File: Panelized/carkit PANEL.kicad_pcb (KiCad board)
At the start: 2 copper layers, 100 x 92 mm, 110 parts, among them J1 Barrel_Jack, J10 Conn_02x03_Odd_Even, J11 Conn_01x02_Pin, J12 Conn_01x02_Pin, J2 Conn_01x02_Pin, J3 Conn_02x03_Odd_Even, J4 Conn_02x03_Odd_Even, J5 Conn_01x02_Pin, J6 Conn_01x02_Pin, J7 Barrel_Jack, J8 Conn_01x02_Pin, J9 Conn_02x03_Odd_Even, P1 USB_C_Plug, P2 USB_C_Plug, SW1 SW_Push, SW2 SW_Push, SW3 SW_Push, SW4 SW_Push, U1 ESP32-C3-MINI-1, U10 DRV8876PWPR, U2 LM2596SX-5.0/NOPB, U3 AMS1117-3.3, U4 DRV8876PWPR, U5 DRV8876PWPR, U6 ESP32-C3-MINI-1, U7 LM2596SX-5.0/NOPB, U8 AMS1117-3.3, U9 DRV8876PWPR

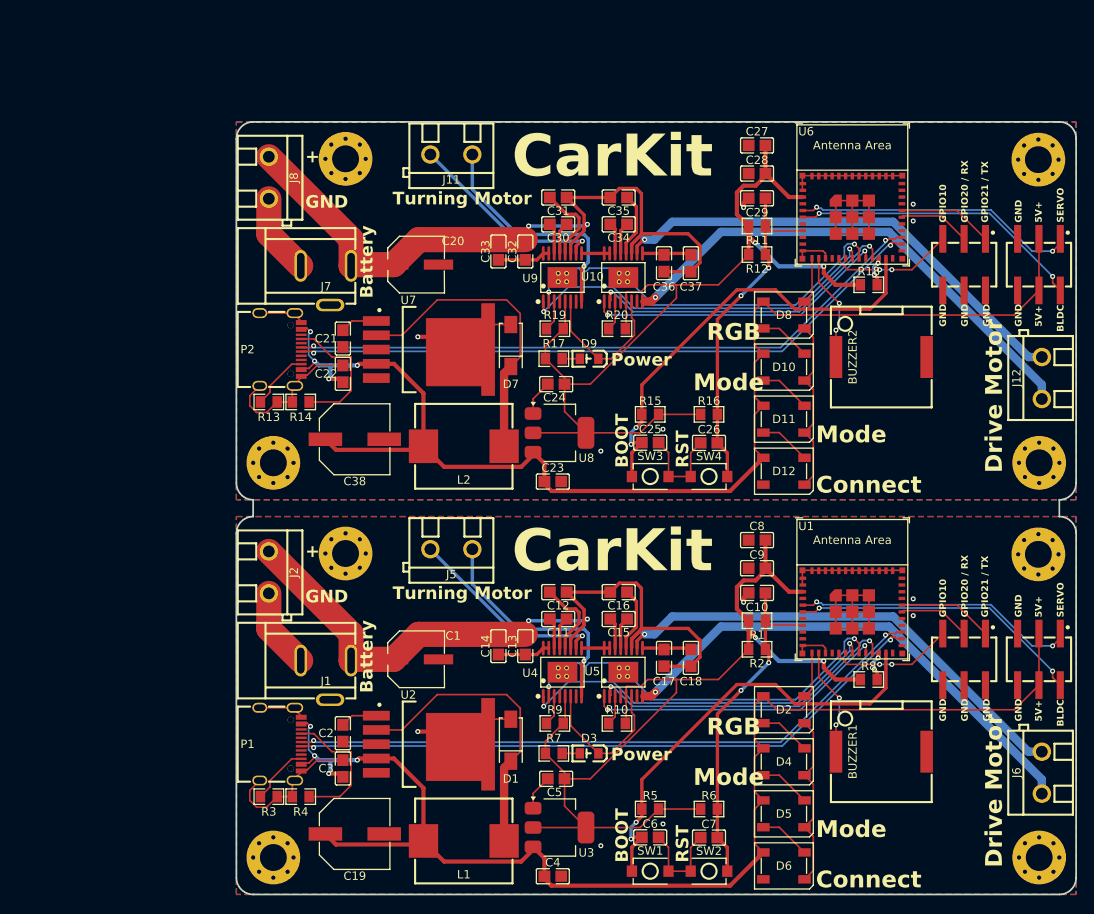
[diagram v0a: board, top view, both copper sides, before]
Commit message: Panelization Complete
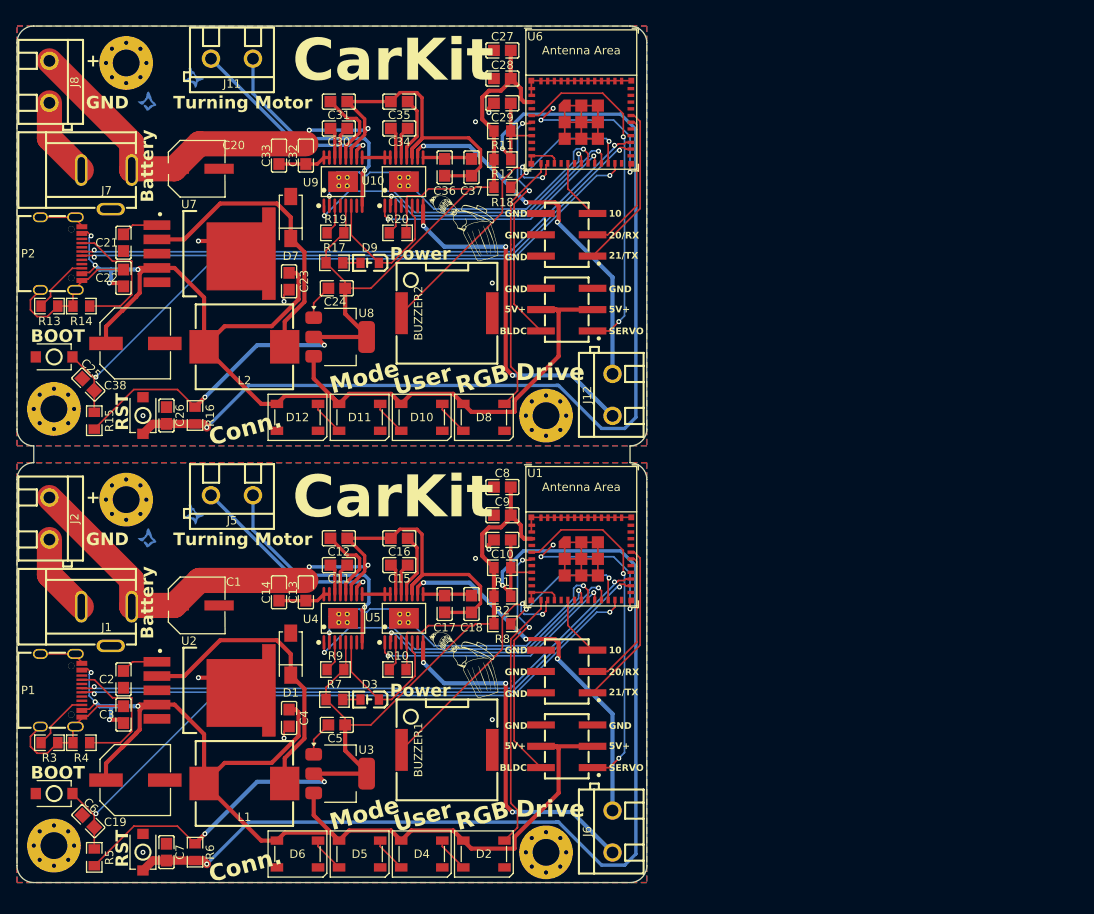
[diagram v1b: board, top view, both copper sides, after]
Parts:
- removed H7, H8: MountingHole, MountingHole:MountingHole_3.2mm_M3_Pad_Via
- added G***: LOGO, LOGO, F.Cu at (117.9, 106.2)
- added G***: LOGO, LOGO, B.Cu at (96.0, 122.6)
- added G***: LOGO, LOGO, B.Cu at (129.3, 94.3)
- added G***: LOGO, LOGO, B.Cu at (102.9, 90.8)
- added G***: LOGO, LOGO, B.Cu at (89.3, 99.5)
- added G***: LOGO, LOGO, B.Cu at (119.6, 114.5)
- added G***: LOGO, LOGO, B.Cu at (115.3, 91.4)
- added G***: LOGO, LOGO, B.Cu at (78.9, 118.2)
- added G***1: LOGO, LOGO, B.Cu at (96.0, 70.6)
- added G***2: LOGO, LOGO, B.Cu at (78.9, 66.2)
- added G***3: LOGO, LOGO, B.Cu at (119.6, 62.5)
- added G***4: LOGO, LOGO, F.Cu at (117.9, 54.2)
- added G***5: LOGO, LOGO, B.Cu at (89.3, 47.5)
- added G***6: LOGO, LOGO, B.Cu at (129.3, 42.3)
- added G***7: LOGO, LOGO, B.Cu at (115.3, 39.4)
- added G***8: LOGO, LOGO, B.Cu at (102.9, 38.8)
- moved H4 128.9 mm to (68.9, 75.4)
- moved SW3 72.4 mm to (69.0, 69.2), turned to 180 degrees
- moved SW1 71.6 mm to (69.0, 121.2), turned to 180 degrees
- moved H3 68.5 mm to (127.5, 128.2)
- moved SW4 67.8 mm to (79.5, 76.1), turned to 90 degrees
- moved SW2 67.4 mm to (79.5, 128.1), turned to 90 degrees
- moved C25 67.3 mm to (73.0, 72.5), turned to 180 degrees
- moved C6 66.9 mm to (73.0, 124.5), turned to 180 degrees
- moved R5 66.5 mm to (73.7, 128.8), turned to 90 degrees
- moved R15 66.2 mm to (73.7, 76.8), turned to 90 degrees
- moved C26 64.7 mm to (82.3, 76.1), turned to 90 degrees
- moved C7 64.6 mm to (82.3, 128.1), turned to 90 degrees
- moved R6 61.4 mm to (85.7, 128.1), turned to -90 degrees
- moved R16 61.2 mm to (85.7, 76.1), turned to -90 degrees
- moved D12 58.3 mm to (97.9, 76.4)
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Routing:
- net CHIP_PU: track 82.0 -> 258.3 mm
- net GPIO 9: track 106.3 -> 161.6 mm
- net LED_DATA: track 11.0 -> 62.2 mm
- net GND: track 324.6 -> 284.9 mm, vias 12 -> 18
- net VCC_5V: track 307.2 -> 267.7 mm
- net M2+: track 120.0 -> 85.6 mm, vias 2 -> 6
- net BUZZER_DATA: track 25.9 -> 58.9 mm
- net M2-: track 113.9 -> 87.2 mm, vias 2 -> 6
- net GPIO 8: track 7.21 -> 33.8 mm
- net GPIO 20: track 17.2 -> 34.3 mm
- net GPIO 21: track 22.7 -> 39.6 mm
- net SERVO_PWM: track 67.9 -> 83.4 mm
- net GPIO 10: track 29.3 -> 14.4 mm, vias 4 -> 0
- net D-: track 154.6 -> 142.2 mm
- net D+: track 154.6 -> 142.2 mm
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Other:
- board size 100 x 92 mm -> 75 x 102 mm
- board text added: "10"
- board text added: "20/RX"
- board text added: "21/TX"
- board text added: "Conn."
- board text added: "Drive"
- board text added: "User"
- board text removed: "Connect"
- board text removed: "Drive Motor"
- board text removed: "GPIO10"
- board text removed: "GPIO20 / RX"
- board text removed: "GPIO21 / TX"
